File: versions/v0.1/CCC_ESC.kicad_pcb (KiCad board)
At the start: 4 copper layers, 100 x 65 mm, 160 parts, among them J1 Conn_01x04, J2 Conn_01x06, J3 Conn_01x06, J4 Conn_01x06, U1 NCP5183, U2 NCP5183, U3 NCP5183, U4 NCS20074D, U5 STM32F401CCU6_Balckpill, U6 PQDE6W-Q110, U7 TO220_replacement_module

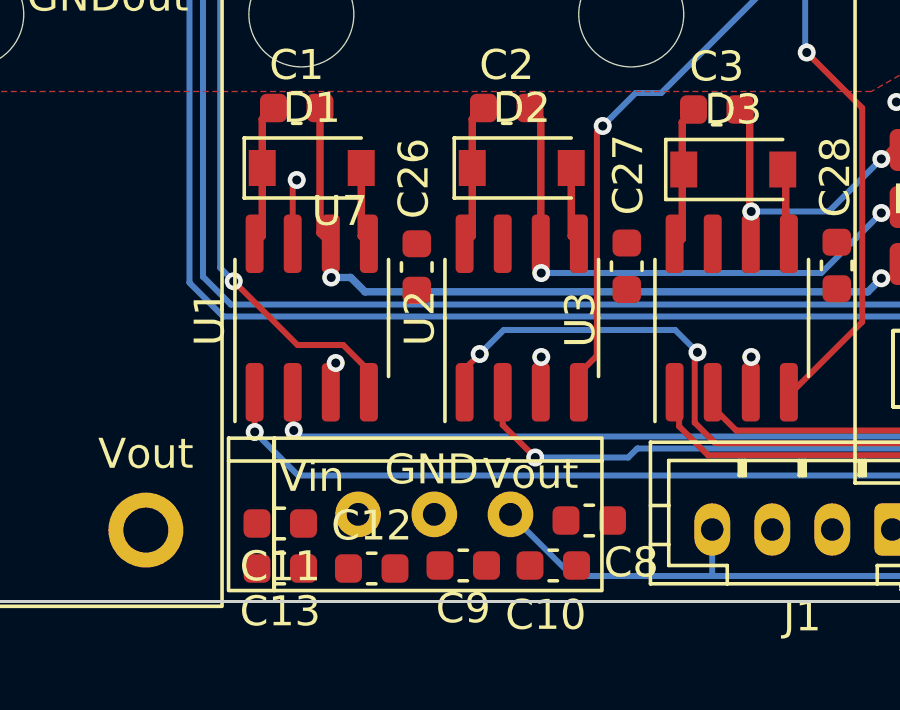
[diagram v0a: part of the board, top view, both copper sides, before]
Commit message: minor thing
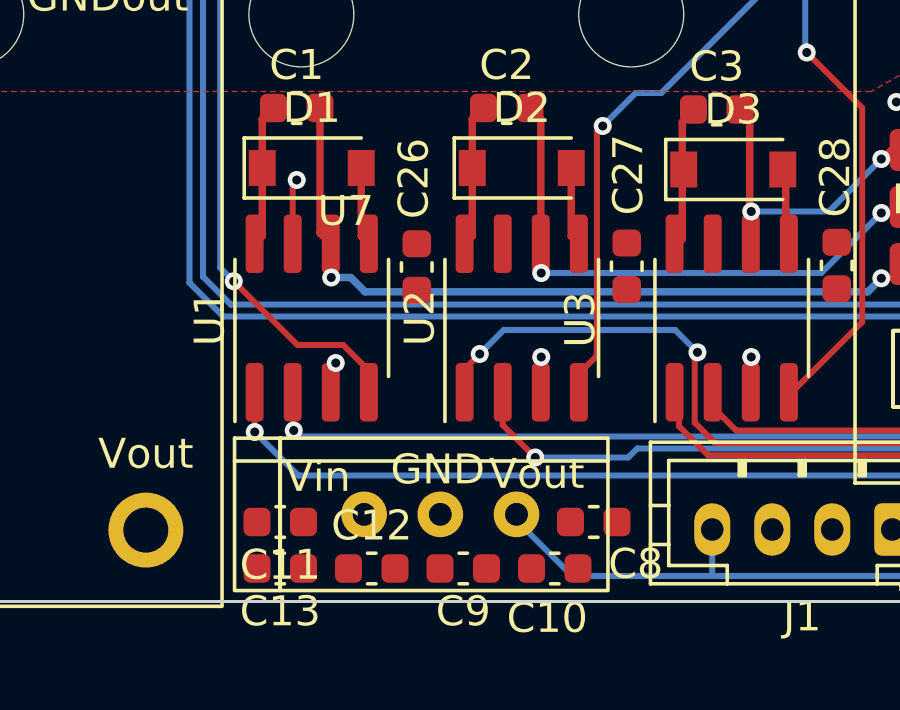
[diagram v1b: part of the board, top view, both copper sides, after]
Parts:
- moved U7 0.20 mm to (77.6, 109.6)
- moved C8 0.16 mm to (87.8, 112.3)
- moved C10 0.11 mm to (86.5, 113.9)
- moved C9 0.10 mm to (83.4, 113.9)
- moved C11 0.05 mm to (77.3, 112.3)
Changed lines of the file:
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@@
   )
   (footprint "Capacitor_SMD:C_0603_1608Metric" (layer "F.Cu")
-    (at 86.4 113.8)
+    (at 86.45 113.9)
     (descr "Capacitor SMD 0603 (1608 Metric), square (rectangular) end terminal, IPC_7351 nominal, (Body size source: IPC-SM-782 page 76, https://www.pcb-3d.com/wordpress/wp-content/uploads/ipc-sm-782a_amendment_1_and_2.pdf), generated with kicad-footprint-generator")
     (tags "capacitor")
@@
   )
   (footprint "CCC_ESC_Custom_parts:TO220_replacement_module" (layer "F.Cu")
-    (at 77.355 109.555)
+    (at 77.555 109.555)
     (property "Sheetfile" "CCC_ESC.kicad_sch")
     (property "Sheetname" "")
@@
   )
   (footprint "Capacitor_SMD:C_0603_1608Metric" (layer "F.Cu")
-    (at 87.6 112.3)
+    (at 87.75 112.35)
     (descr "Capacitor SMD 0603 (1608 Metric), square (rectangular) end terminal, IPC_7351 nominal, (Body size source: IPC-SM-782 page 76, https://www.pcb-3d.com/wordpress/wp-content/uploads/ipc-sm-782a_amendment_1_and_2.pdf), generated with kicad-footprint-generator")
     (tags "capacitor")
@@
   )
   (footprint "Capacitor_SMD:C_0603_1608Metric" (layer "F.Cu")
-    (at 77.3 112.4 180)
+    (at 77.3 112.35 180)
     (descr "Capacitor SMD 0603 (1608 Metric), square (rectangular) end terminal, IPC_7351 nominal, (Body size source: IPC-SM-782 page 76, https://www.pcb-3d.com/wordpress/wp-content/uploads/ipc-sm-782a_amendment_1_and_2.pdf), generated with kicad-footprint-generator")
     (tags "capacitor")
@@
   )
   (footprint "Capacitor_SMD:C_0603_1608Metric" (layer "F.Cu")
-    (at 83.4 113.8 180)
+    (at 83.4 113.9 180)
     (descr "Capacitor SMD 0603 (1608 Metric), square (rectangular) end terminal, IPC_7351 nominal, (Body size source: IPC-SM-782 page 76, https://www.pcb-3d.com/wordpress/wp-content/uploads/ipc-sm-782a_amendment_1_and_2.pdf), generated with kicad-footprint-generator")
     (tags "capacitor")
